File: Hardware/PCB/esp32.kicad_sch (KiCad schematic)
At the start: 10 parts, among them J18 Programmer, U11 ESP32-S3-WROOM-1U-N16R8

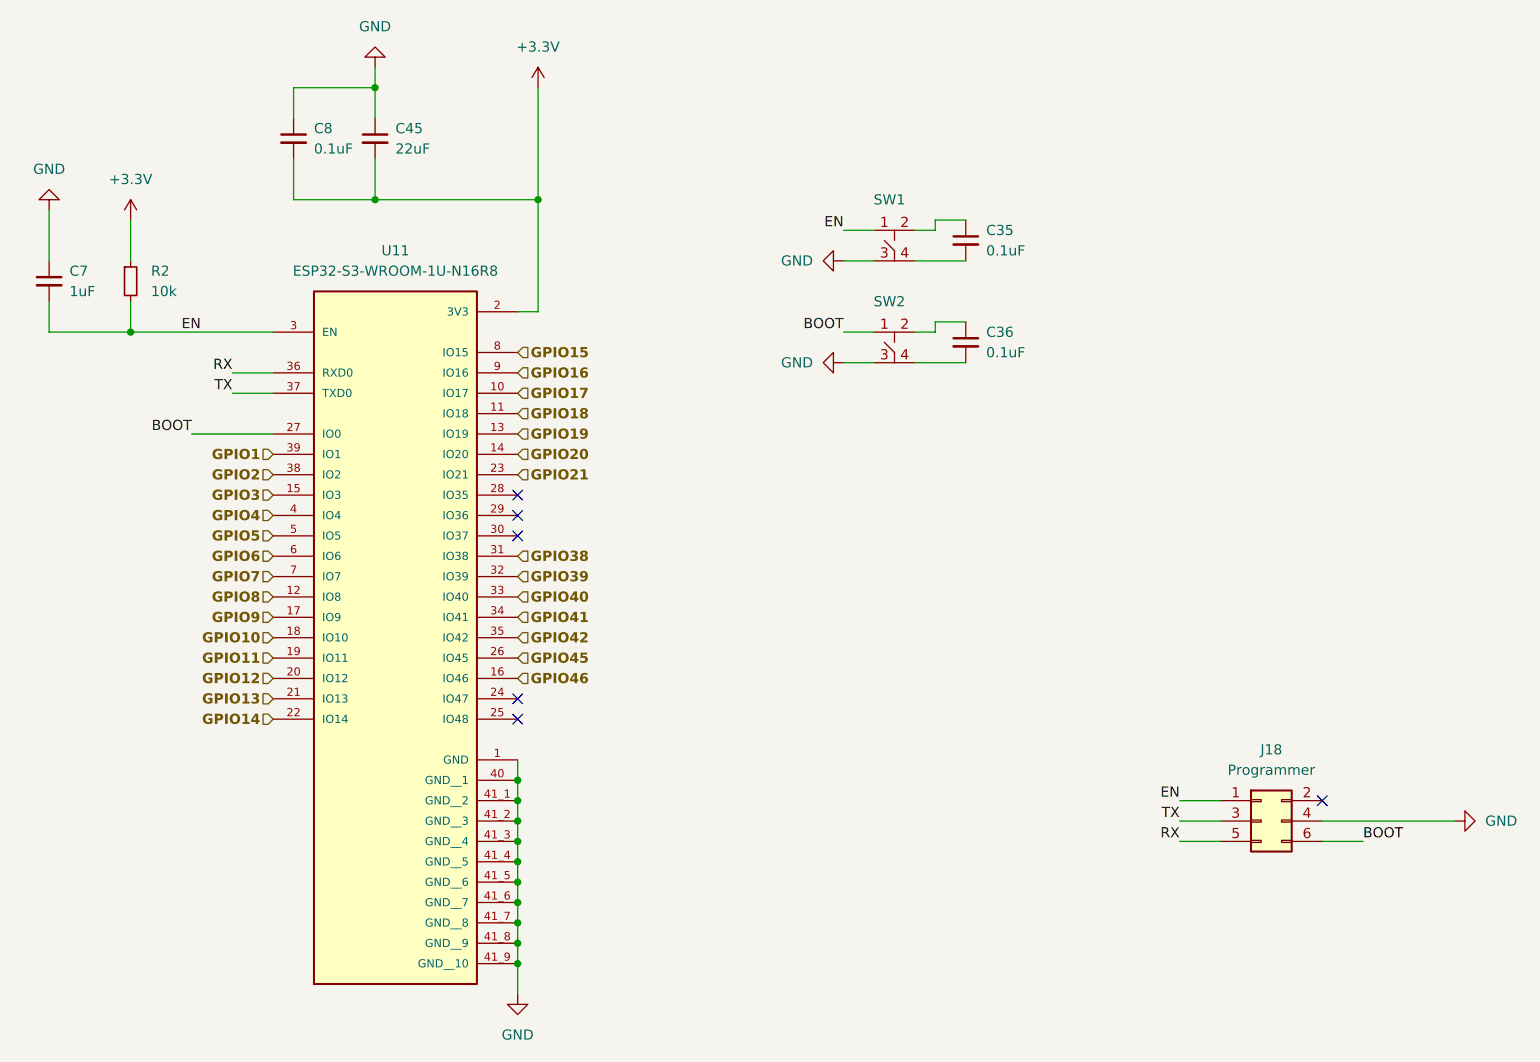
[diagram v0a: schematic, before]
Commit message: kinda pricey, I should try to make a smaller version using LCSC parts for cheaper solution
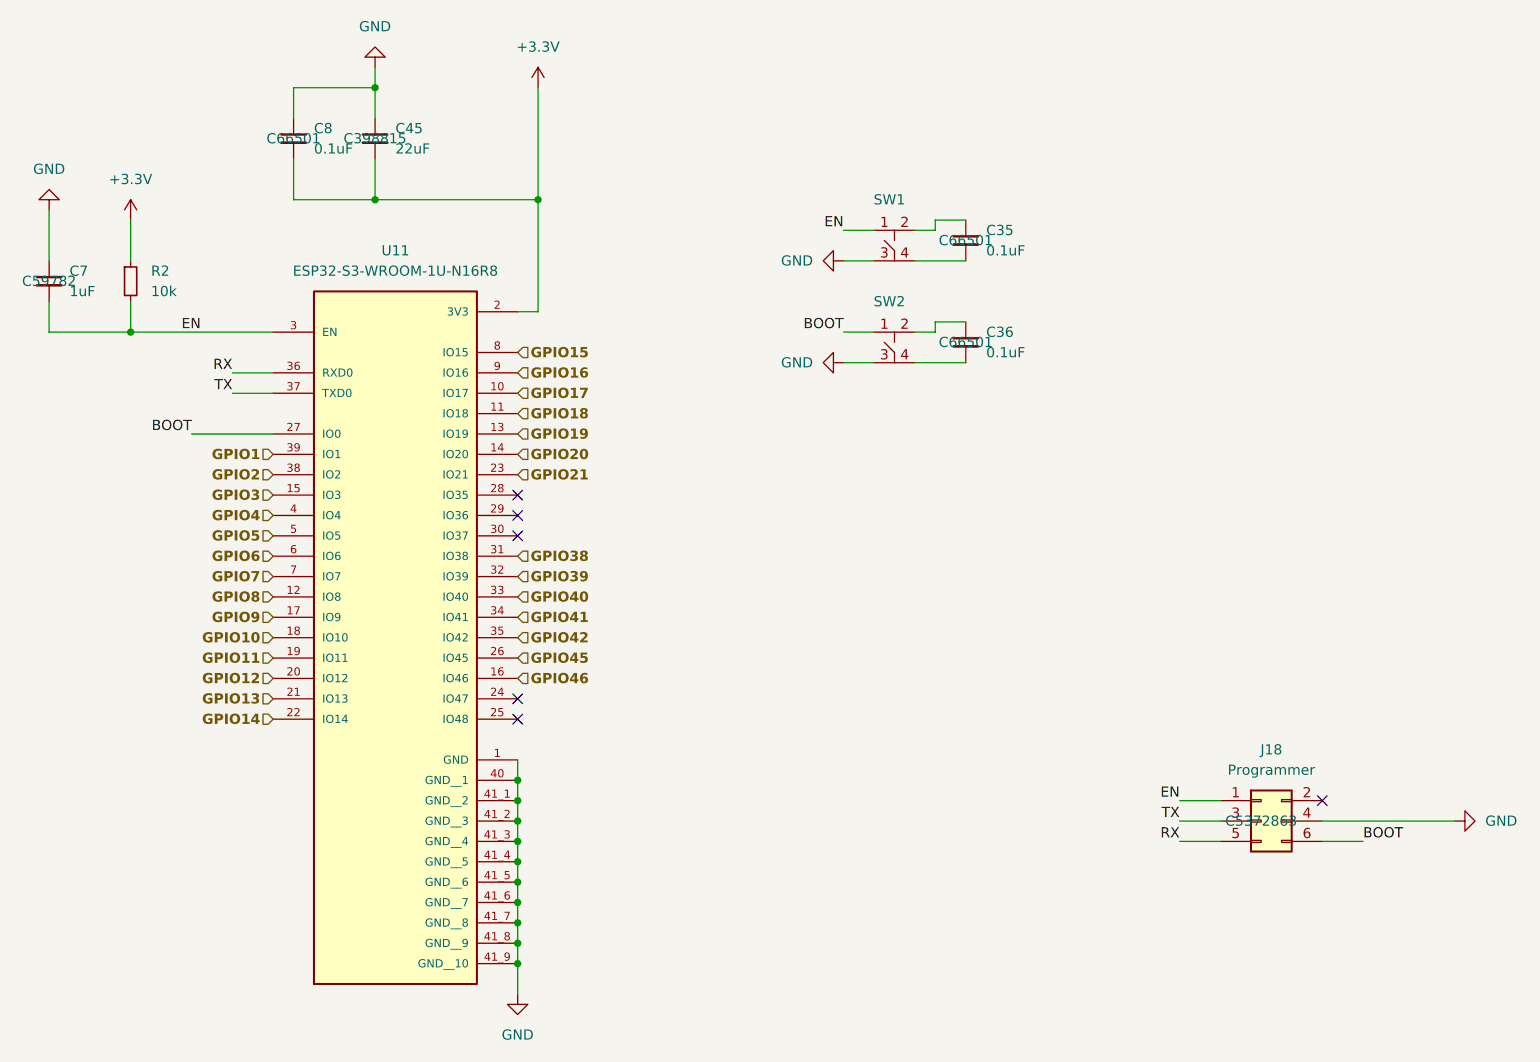
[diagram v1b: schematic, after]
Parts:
- C35, C36, C8: LCSC (none) -> C66501
- C45: LCSC (none) -> C398815
- C7: LCSC (none) -> C59782
- J18: LCSC (none) -> C5372863
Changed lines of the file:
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@@
+			)
+		)
+		(property "LCSC" "C66501"
+			(at 157.48 64.77 0)
+			(effects
+				(font
+					(size 1.27 1.27)
+				)
 			)
 		)
@@
 			)
 		)
+		(property "LCSC" ""
+			(at 53.34 69.85 0)
+			(effects
+				(font
+					(size 1.27 1.27)
+				)
+			)
+		)
 		(pin "1"
 		)
@@
 			)
 		)
+		(property "LCSC" ""
+			(at 148.59 63.5 0)
+			(effects
+				(font
+					(size 1.27 1.27)
+				)
+			)
+		)
 		(pin "3"
 		)
@@
 			)
 		)
+		(property "LCSC" "C59782"
+			(at 43.18 69.85 0)
+			(effects
+				(font
+					(size 1.27 1.27)
+				)
+			)
+		)
 		(pin "2"
 		)
@@
 			)
 		)
+		(property "LCSC" "C398815"
+			(at 83.82 52.07 0)
+			(effects
+				(font
+					(size 1.27 1.27)
+				)
+			)
+		)
 		(pin "2"
 		)
@@
 			)
 		)
+		(property "LCSC" ""
+			(at 86.36 101.6 0)
+			(effects
+				(font
+					(size 1.27 1.27)
+				)
+			)
+		)
 		(pin "9"
 		)
@@
 			)
 		)
+		(property "LCSC" "C5372863"
+			(at 194.31 137.16 0)
+			(effects
+				(font
+					(size 1.27 1.27)
+				)
+			)
+		)
 		(pin "2"
 		)
@@
 			)
 		)
+		(property "LCSC" "C66501"
+			(at 157.48 77.47 0)
+			(effects
+				(font
+					(size 1.27 1.27)
+				)
+			)
+		)
 		(pin "2"
 		)
@@
 			)
 		)
+		(property "LCSC" "C66501"
+			(at 73.66 52.07 0)
+			(effects
+				(font
+					(size 1.27 1.27)
+				)
+			)
+		)
 		(pin "2"
 		)
@@
 			)
 		)
+		(property "LCSC" ""
+			(at 148.59 76.2 0)
+			(effects
+				(font
+					(size 1.27 1.27)
+				)
+			)
+		)

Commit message: done with this, placed order
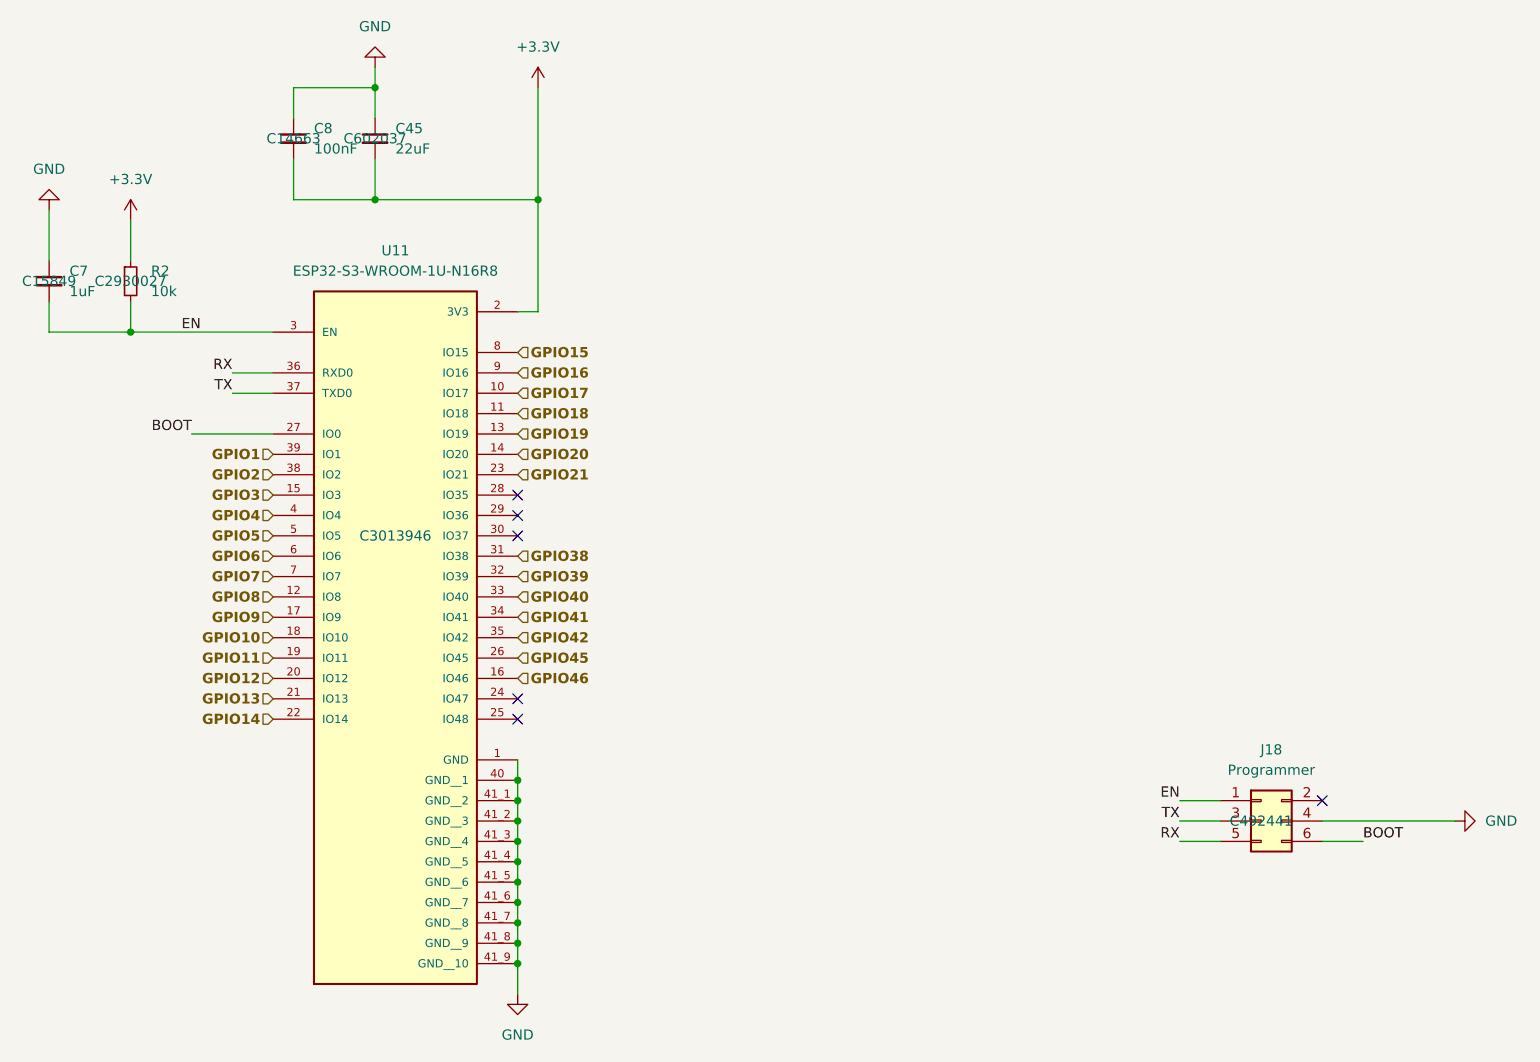
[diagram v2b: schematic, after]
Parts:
- removed C35, C36: 0.1uF, Capacitor_SMD:C_0603_1608Metric_Pad1.08x0.95mm_HandSolder, symbol Device:C_Small
- removed SW1, SW2: ~, Vendor_Footprints:PTS647SN50SMTR2LFS, symbol Vendor_Symbols:PTS647SN50SMTR2_LFS
- C45: LCSC C398815 -> C602037; MPN CL21A226MOCLRNC -> CL21A226MAYNNNE
- C7: LCSC C59782 -> C15849; MPN CL10B105KO8NNNC -> CL10A105KB8NNNC
- C8: value 0.1uF -> 100nF; LCSC C66501 -> C14663; MPN CL10B104KO8NNNC -> CC0603KRX7R9BB104; Manufacturer Samsung Electro-Mechanics -> YAGEO
- J18: DigiKey Link https://www.digikey.com/en/products/detail/w%C3%BCrth-elekt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 -> (none); LCSC C5372863 -> C492441; MPN 61200621621 -> XFCN BH254V-6P; Manufacturer Würth Elektronik -> XFCN
- R2: LCSC (none) -> C2930027; MPN RMCF0603JT10K0 -> FRC0603J103TS; Manufacturer Stackpole Electronics Inc -> FOJAN
- U11: DigiKey Link https://www.digikey.com/en/products/detail/espressif-system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 -> (none); LCSC (none) -> C3013946
